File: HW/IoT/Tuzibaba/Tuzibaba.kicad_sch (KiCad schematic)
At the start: 7 parts, among them J1 2x9 2.54mm 90deg female, J2 1x5 2.54mm male

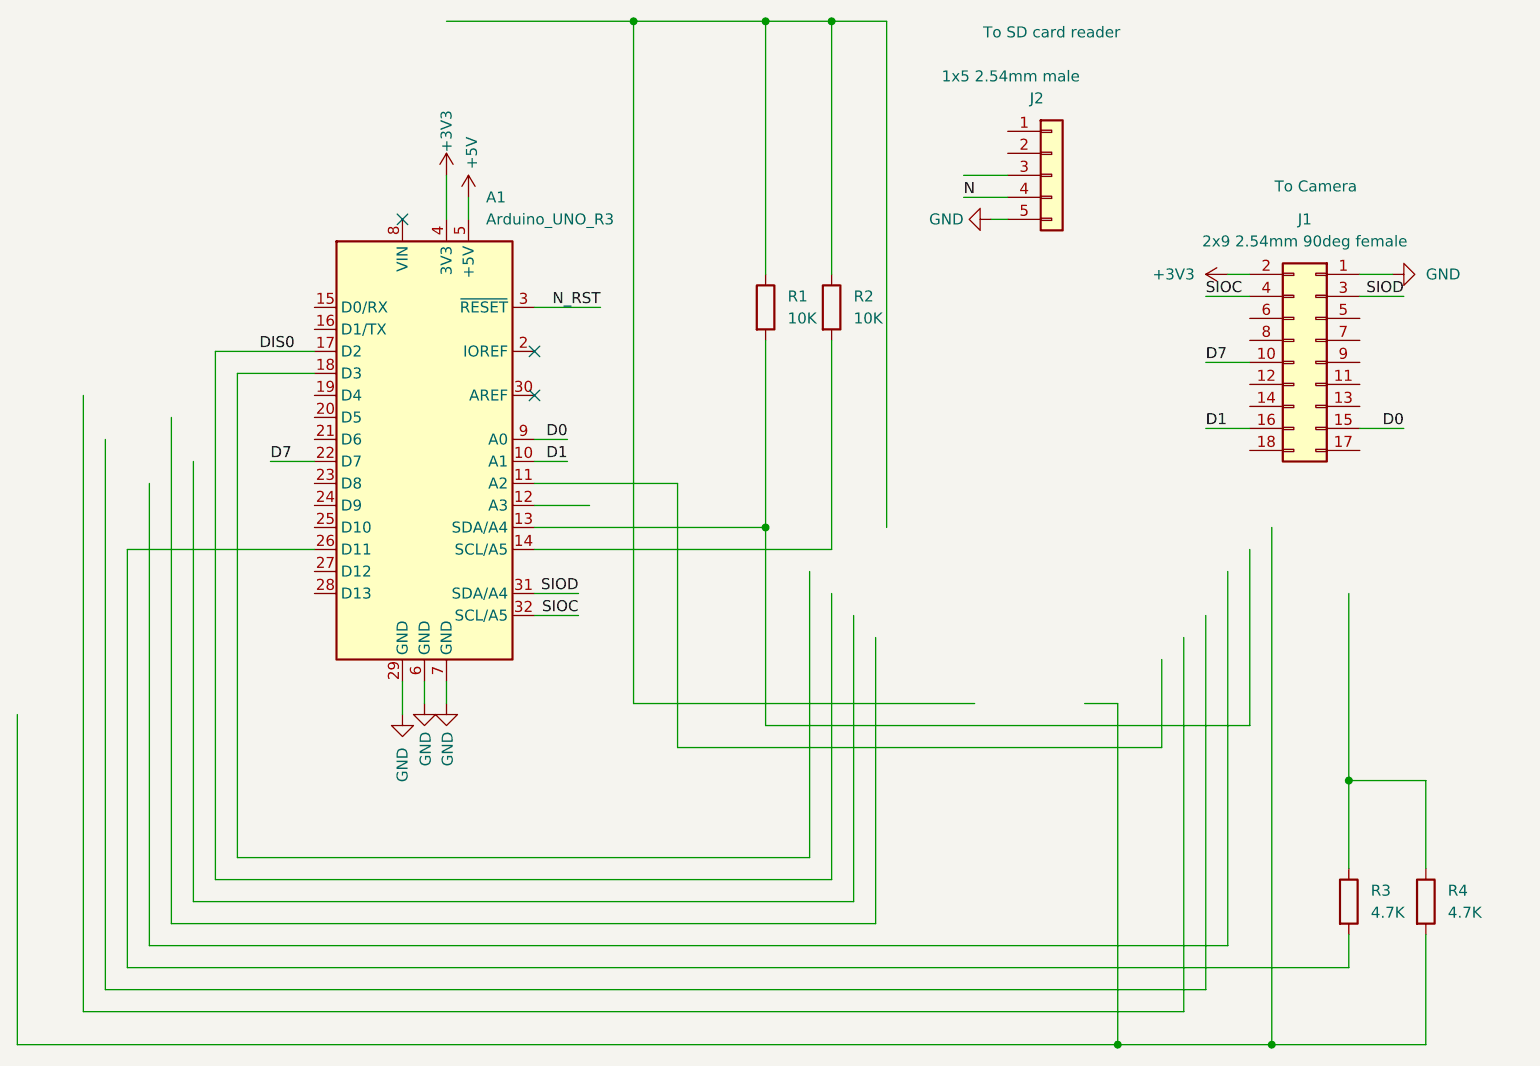
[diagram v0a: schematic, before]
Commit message: Finalizing schematic
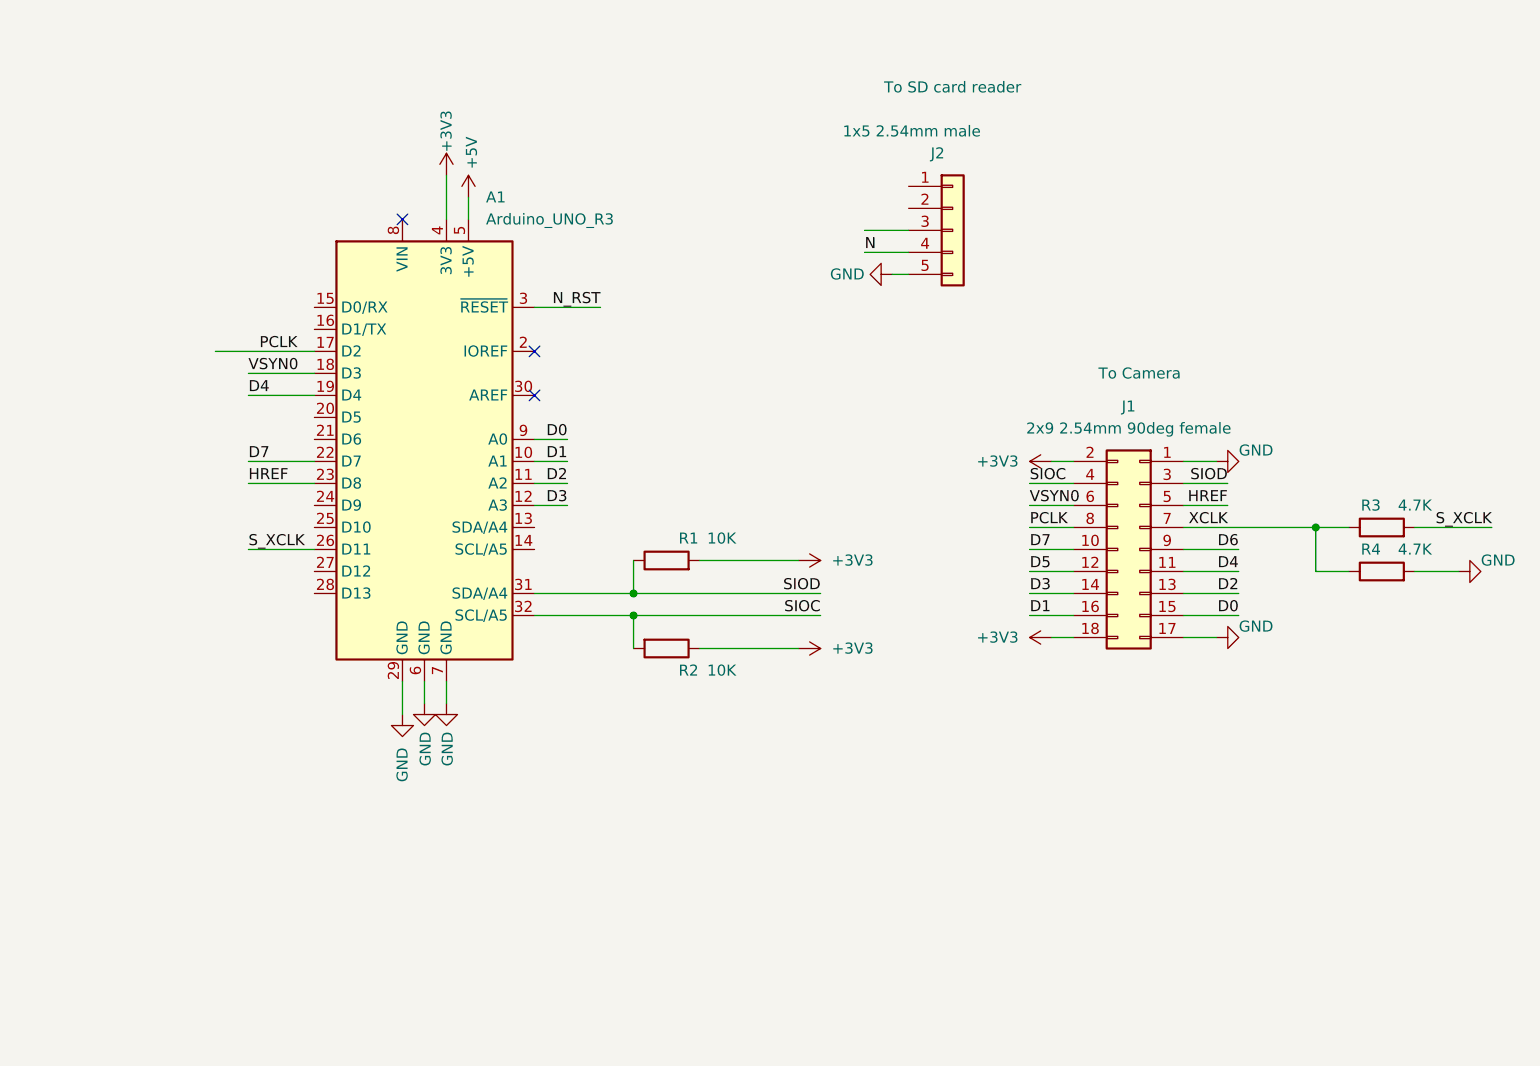
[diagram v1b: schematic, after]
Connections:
- net DIS0 is gone; now on net PCLK: A1.17 (D2)
- net +3V3: now also J1.18 (Pin_18), R1.2, R2.1
- net GND: now also J1.17 (Pin_17), R4.2
- net SIOC: now also R2.2
- net SIOD: now also R1.1
- net XCLK: now reaches R3.1, R4.1
- net XCLK: now also J1.7 (Pin_7)
- net S_XCLK: now reaches A1.26 (D11), R3.2
- net D2: now reaches A1.11 (A2)
- net D2: now also J1.13 (Pin_13)
- net D3: now reaches A1.12 (A3)
- net D3: now also J1.14 (Pin_14)
- net at A1.13 (SDA/A4): no longer R1.2
- net at A1.14 (SCL/A5): no longer R2.2
- net VSYN0: now reaches A1.18 (D3)
- net VSYN0: now also J1.6 (Pin_6)
- net D4: now reaches A1.19 (D4)
- net D4: now also J1.11 (Pin_11)
- net HREF: now reaches A1.23 (D8)
- net HREF: now also J1.5 (Pin_5)
- net D5: now reaches J1.12 (Pin_12)
- net PCLK: now reaches J1.8 (Pin_8)
- net D6: now reaches J1.9 (Pin_9)
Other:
- moved on the sheet: J1, J2, R1, R2, R3, R4
